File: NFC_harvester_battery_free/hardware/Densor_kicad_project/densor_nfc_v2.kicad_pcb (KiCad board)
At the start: 2 copper layers, 46.4 x 18.8 mm, 27 parts, among them J1 Conn_ARM_JTAG_SWD_10, J2 Conn_01x08_Pin, J3 Conn_01x04_Pin, U1 ST25DV04K-JFR6D3, U2 AM1805, U3 MAX30208CLB+, U4 STM32L011F3Ux, U5 LIS2DW12, U6 TS3A44159, Y1 Crystal

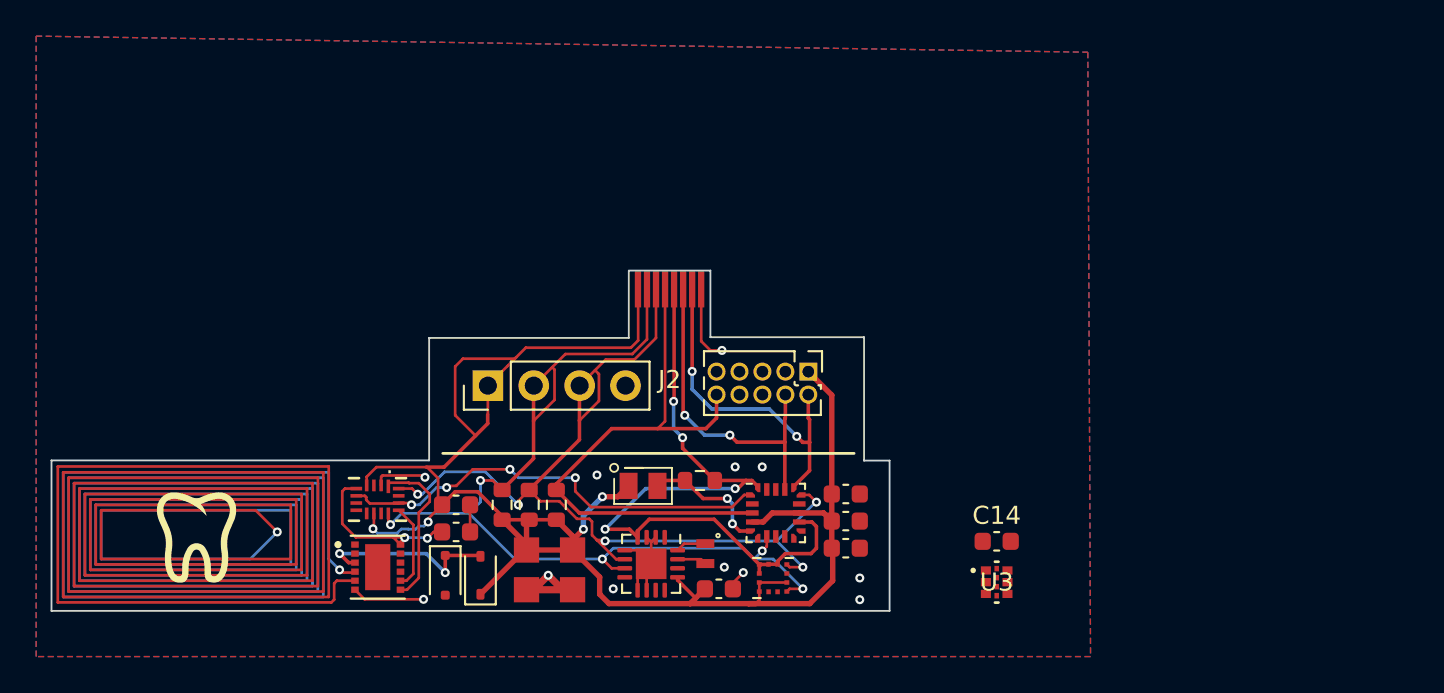
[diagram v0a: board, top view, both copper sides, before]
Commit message: Schemetics and PCB layout finished
Concept diagram added
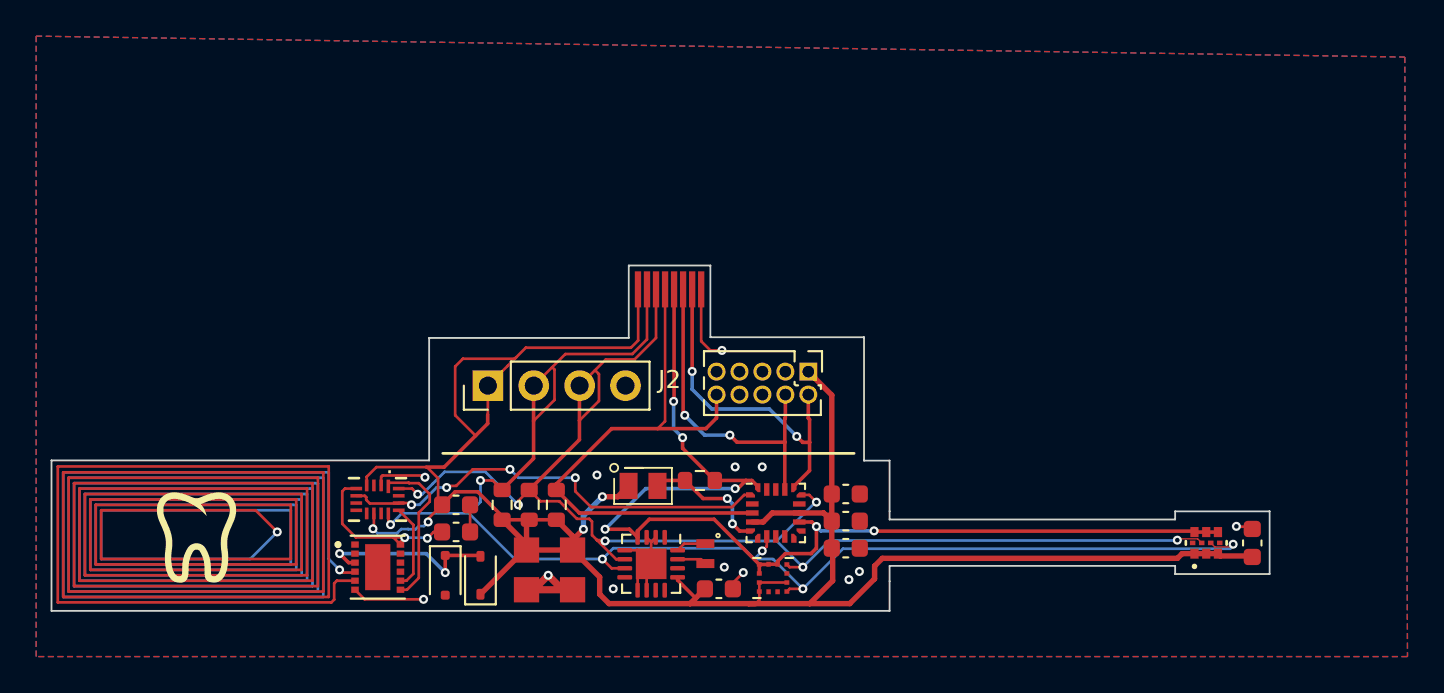
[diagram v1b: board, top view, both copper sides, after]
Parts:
- moved C14 14.2 mm to (186.6, 94.4), turned to 90 degrees
- moved U3 11.8 mm to (184.0, 94.4), turned to 90 degrees
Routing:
- net /i2c_scl: track 53.5 -> 79.9 mm, vias 5 -> 6
- net /V_MCU: track 103.0 -> 129.1 mm
- net /i2c_sda: track 51.7 -> 74.6 mm, vias 5 -> 6
- net /PSW: track 39.7 -> 62.2 mm, vias 4 -> 6
- net GND: track 26.7 -> 27.7 mm, vias 12 -> 13
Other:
- board size 46.4 x 18.8 mm -> 67.4 x 19.1 mm
